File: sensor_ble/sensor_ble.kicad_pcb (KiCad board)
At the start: 2 copper layers, 30.5 x 21.6 mm, 28 parts, among them U1 Nrf52810-QCAA, U2 BME280, Y1 32,768KHz, Y2 32MHz

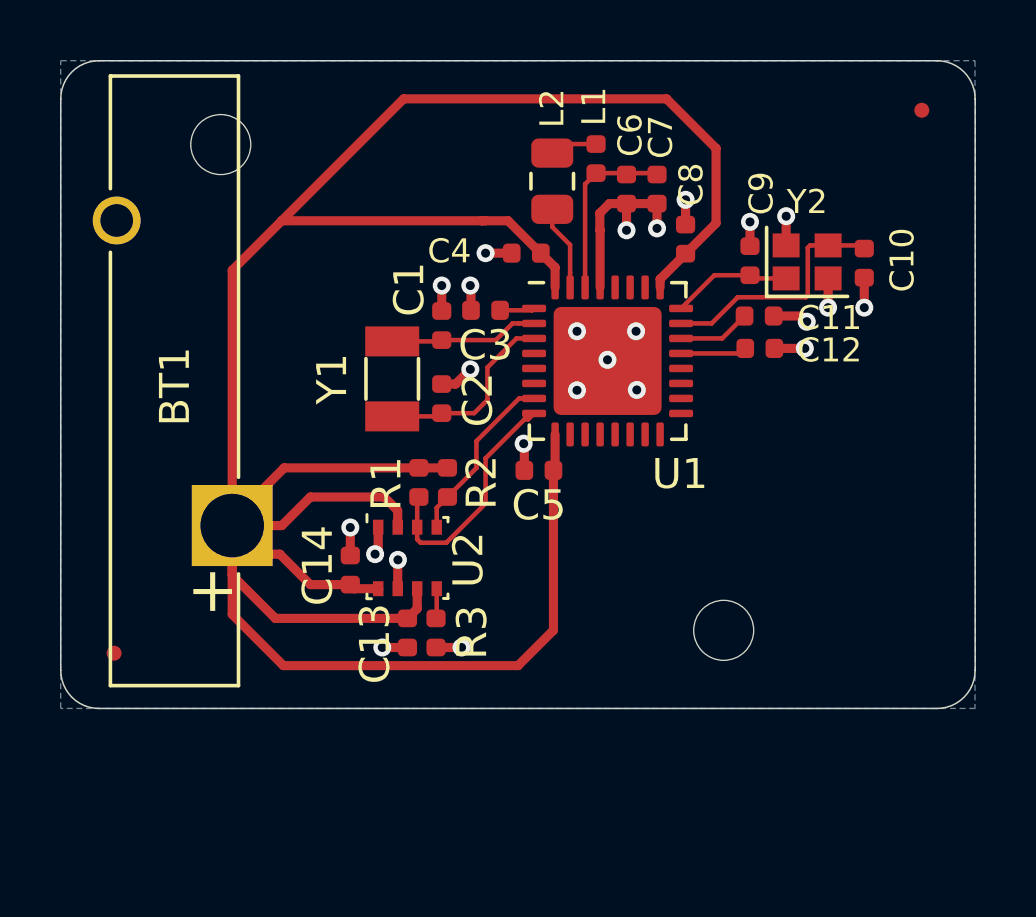
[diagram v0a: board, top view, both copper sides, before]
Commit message: Adiciona antena
Signed-off-by: Rodrigo Peixoto <rodrigopex@ic.ufal.br>
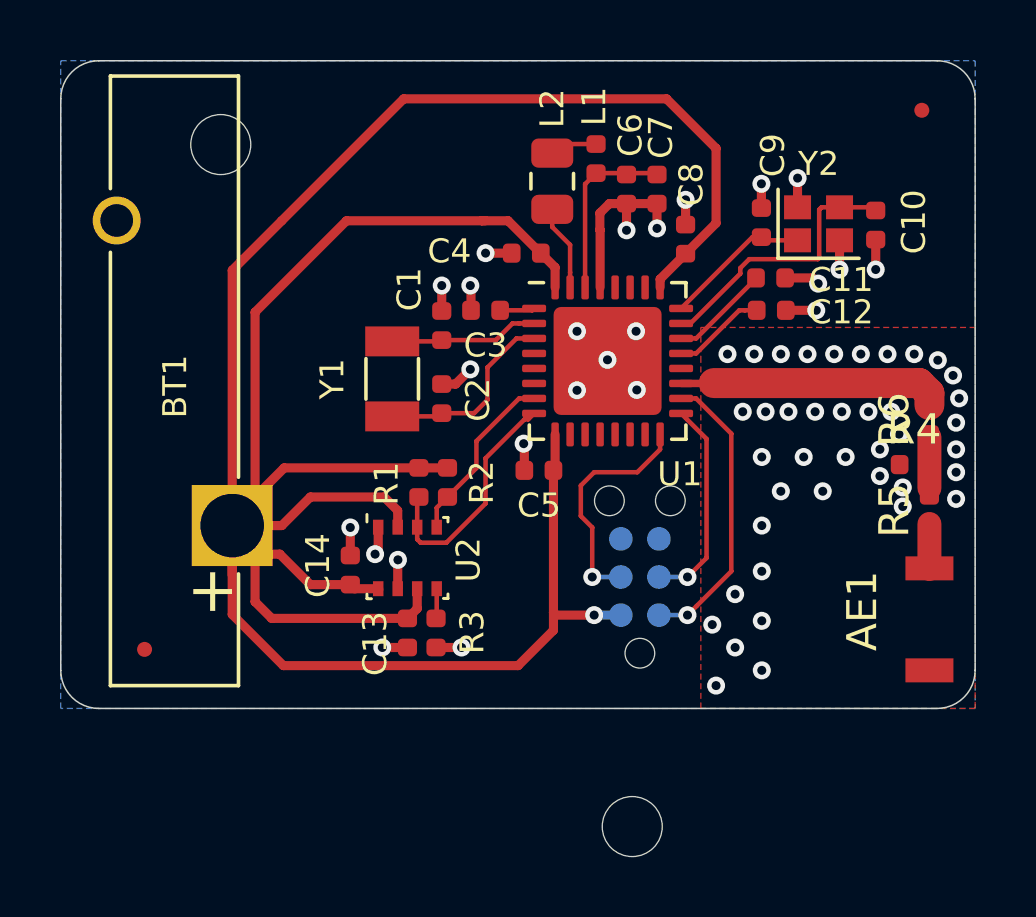
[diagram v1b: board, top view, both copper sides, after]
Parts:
- added AE1: Antenna_Chip, sensor_ble:2450AT18B100, F.Cu at (112.8, 98.6)
- added J1: TC2030, Connector:Tag-Connect_TC2030-IDC-NL_2x03_P1.27mm_Vertical, B.Cu at (103.1, 97.2)
- added R4: NC, Resistor_SMD:R_0402_1005Metric, F.Cu at (112.3, 93.5)
- added R5: 0, Resistor_SMD:R_0402_1005Metric, F.Cu at (112.8, 95.0)
- added R6: NC, Resistor_SMD:R_0402_1005Metric, F.Cu at (112.8, 92.0)
- moved H2 7.22 mm to (102.9, 105.5)
- moved C10 1.33 mm to (111.0, 85.5)
- moved C11 1.33 mm to (107.5, 87.2)
- moved C12 1.33 mm to (107.5, 88.3)
- moved Y2 1.33 mm to (109.1, 85.4)
- moved C9 1.33 mm to (107.2, 85.4)
- moved FID1 1.02 mm to (86.6, 99.6)
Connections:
- U1 pad 16: (no net) -> /NRESET
- U1 pad 17: (no net) -> /SWCLK
- U1 pad 18: (no net) -> /SWDIO
- U1 pad 19: (no net) -> /ANT
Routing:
- net VDD: track 95.9 -> 109.5 mm, vias 0 -> 1
- net /SWDIO: track 0.00 -> 9.77 mm, vias 0 -> 1
- net /ANT: track 0.00 -> 8.36 mm
- net /NRESET: track 0.00 -> 7.80 mm, vias 0 -> 1
- net /SWCLK: track 0.00 -> 7.02 mm, vias 0 -> 1
- net Net-(R4-Pad2): track 0.00 -> 1.70 mm
- net Net-(AE1-Pad1): track 0.00 -> 1.50 mm
- net Net-(C10-Pad2): track 8.15 -> 9.18 mm
- net Net-(C11-Pad2): track 2.43 -> 3.34 mm
- net Net-(C12-Pad2): track 2.21 -> 3.12 mm
- net Net-(C9-Pad2): track 4.00 -> 4.91 mm
- net GND: vias 24 -> 64
- added copper zone on F.Cu, net GND
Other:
- net class ANT added: clearance 0.1524, trace_width 1, via_dia 0.6, via_drill 0.3

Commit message: Últimas mudanças
Signed-off-by: Rodrigo Peixoto <rodrigopex@ic.ufal.br>
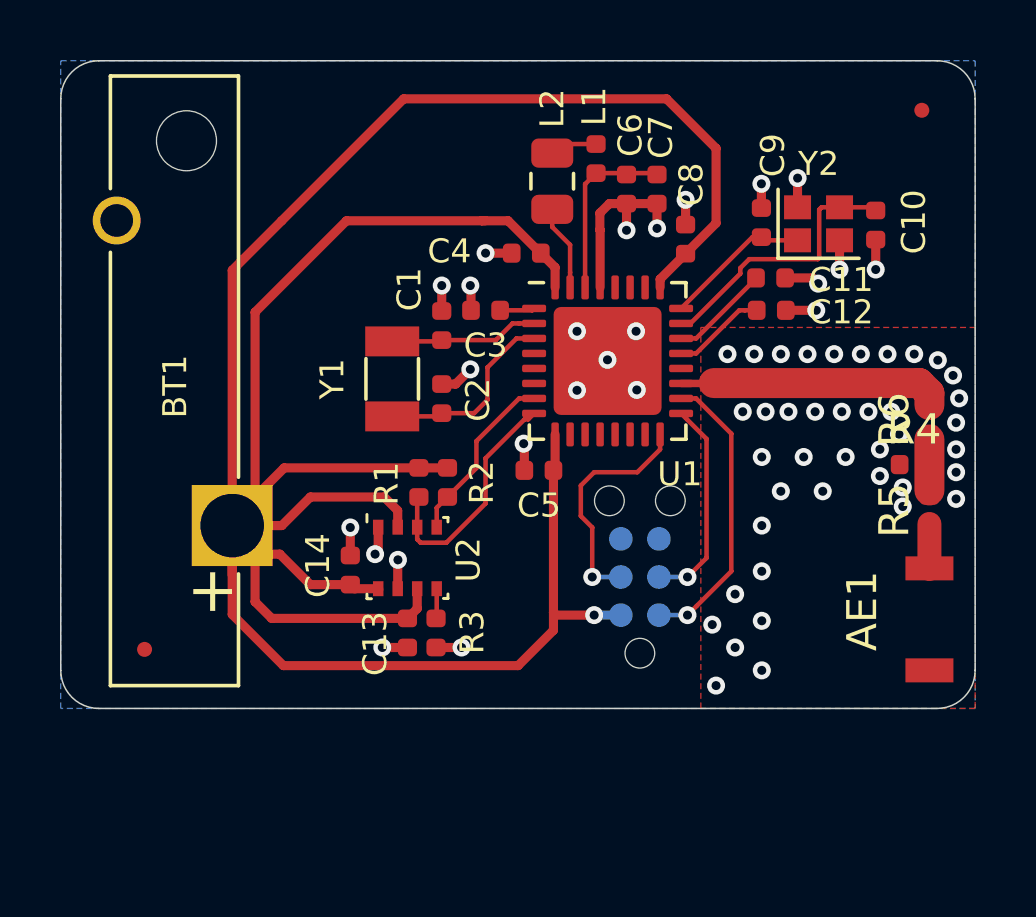
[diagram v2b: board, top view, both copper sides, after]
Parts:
- removed H2: MountingHole, MountingHole:MountingHole_2mm
- moved H1 1.15 mm to (88.0, 82.7)
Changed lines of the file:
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@@
     (tracks 244)
     (zones 0)
-    (modules 33)
+    (modules 32)
     (nets 22)
   )
@@
     (visible_elements FFFFFF7F)
     (pcbplotparams
-      (layerselection 0x010fc_ffffffff)
-      (usegerberextensions false)
+      (layerselection 0x011f8_ffffffff)
+      (usegerberextensions true)
       (usegerberattributes false)
       (usegerberadvancedattributes false)
@@
       (outputformat 1)
       (mirror false)
-      (drillshape 1)
+      (drillshape 0)
       (scaleselection 1)
-      (outputdirectory ""))
+      (outputdirectory "gerbers/"))
   )
   (net 0 "")
@@
   )
   (module MountingHole:MountingHole_2mm (layer F.Cu)
-    (at 102.87 105.537)
-    (descr "Mounting Hole 2mm, no annular")
-    (tags "mounting hole 2mm no annular")
-    (attr virtual)
-    (fp_text reference H2 (at 0 -3.2) (layer F.SilkS) hide
-      (effects (font (size 0.8 0.8) (thickness 0.15)))
-    )
-    (fp_text value MountingHole (at 0 3.1) (layer F.Fab)
-      (effects (font (size 0.8 0.8) (thickness 0.15)))
-    )
-    (fp_circle (center 0 0) (end 2.25 0) (layer F.CrtYd) (width 0.05))
-    (fp_circle (center 0 0) (end 2 0) (layer Cmts.User) (width 0.15))
-    (fp_text user %R (at 0.3 0) (layer F.Fab)
-      (effects (font (size 0.8 0.8) (thickness 0.15)))
-    )
-    (pad "" np_thru_hole circle (at 0 0) (size 2 2) (drill 2) (layers *.Cu *.Mask))
-  )
-  (module MountingHole:MountingHole_2mm (layer F.Cu)
-    (at 89.154 82.804)
+    (at 88.011 82.677)
     (descr "Mounting Hole 2mm, no annular")
     (tags "mounting hole 2mm no annular")
@@
   (segment (start 112.776 91.486) (end 112.776 91.091) (width 1) (layer F.Cu) (net 20))
   (segment (start 112.4392 90.7542) (end 105.5878 90.7542) (width 1) (layer F.Cu) (net 20))
-  (segment (start 112.776 92.556) (end 112.776 94.257) (width 0.8) (layer F.Cu) (net 21))
+  (segment (start 112.776 92.6338) (end 112.776 94.3348) (width 1) (layer F.Cu) (net 21))
   (zone (net 1) (net_name GND) (layer B.Cu) (hatch edge 0.508)
     (connect_pads thru_hole_only (clearance 0.1524))
